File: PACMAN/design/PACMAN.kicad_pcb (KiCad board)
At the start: 2 copper layers, 47 x 57.2 mm, 8 parts, among them P1 RPi connector, P2 CO2, P3 DHT22, P4 Sonar, P5 PMS3003

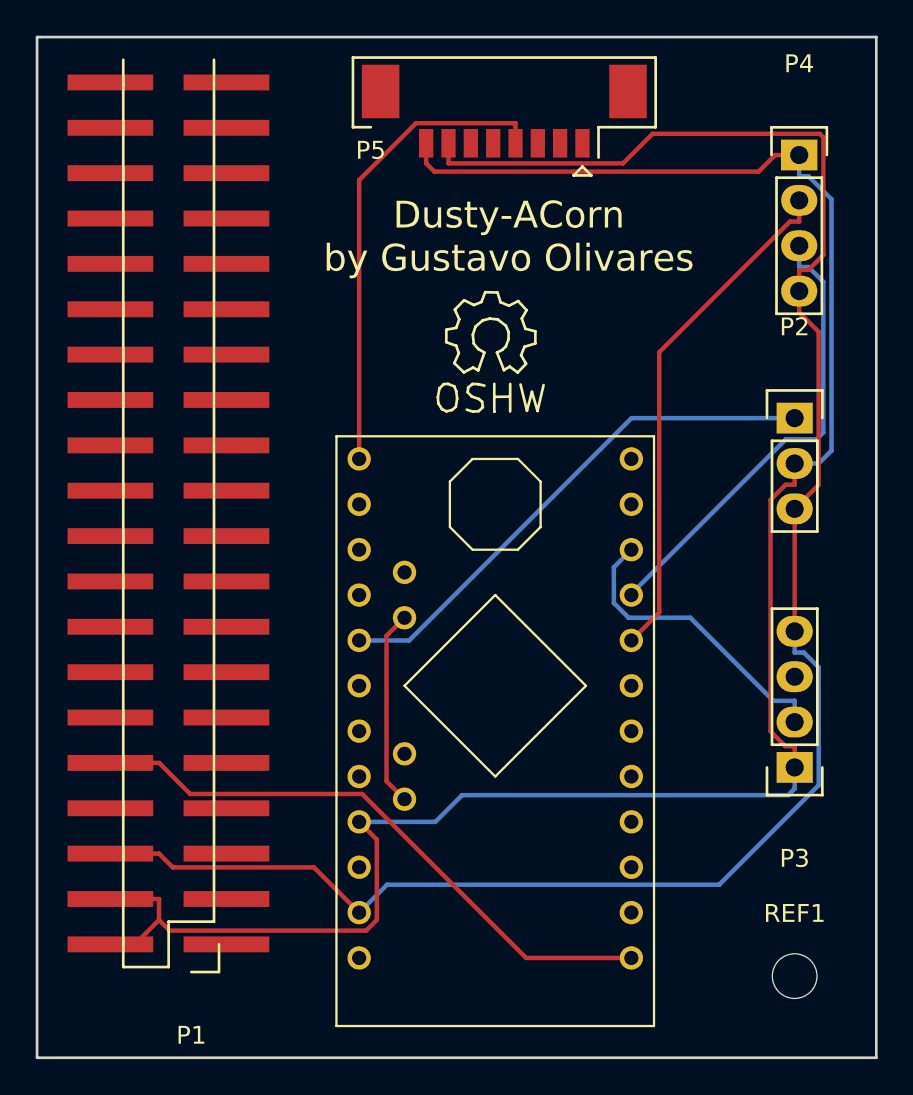
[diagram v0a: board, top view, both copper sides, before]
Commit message: Merging work at work to prepare deployment
Signed-off-by: Gustavo Olivares <guolivar@gmail.com>
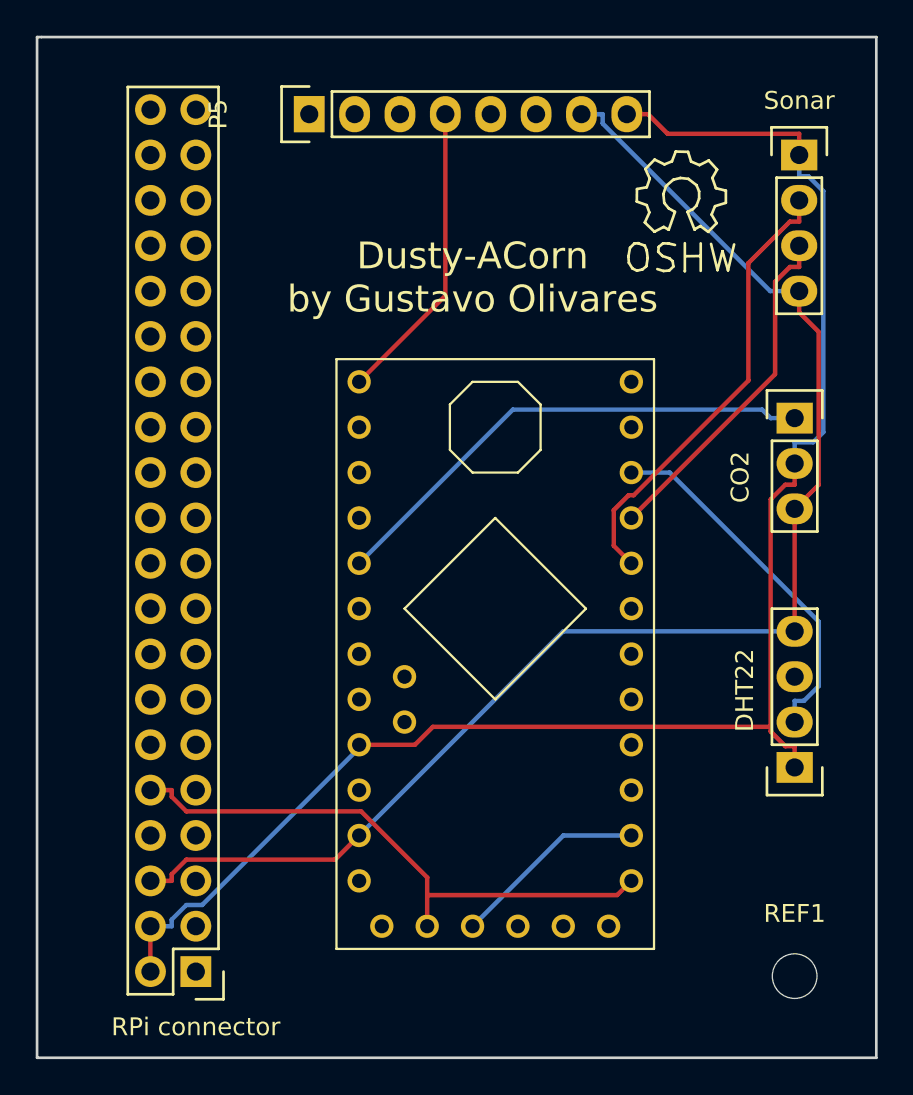
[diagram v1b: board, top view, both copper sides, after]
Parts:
- removed ??1: ARDUINO_PRO_MINI, arduino_pro_mini_V2:Halley-ARDUINO_PRO_MINI
- added MC1: ARDUINO_PRO_MINI, arduino:Halley-ARDUINO_PRO_MINI, F.Cu at (116.3, 111.5)
- P1: footprint headers:Pin_Header_Straight_2x20_SMD -> Pin_Headers:Pin_Header_Straight_2x20
- P5: footprint Connectors_Molex:Connector_Molex_PicoBlade_53261-0871 -> Pin_Headers:Pin_Header_Straight_1x08
- moved REF2 13.3 mm to (126.7, 84.6)
- moved P5 11.0 mm to (105.9, 80.0), turned to 90 degrees
- moved P1 1.55 mm to (99.6, 128.0)
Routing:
- net GND: track 105.9 -> 78.7 mm
- net +5V: track 113.4 -> 91.7 mm
- net Net-(??1-PadA5): track 11.0 -> 0.00 mm
- net Net-(MC1-PadRXI): track 0.00 -> 11.0 mm
- net /D10: track 26.8 -> 17.0 mm
- net /D6: track 25.9 -> 19.4 mm
- net /D7: track 17.0 -> 20.4 mm
- net /D5: track 28.8 -> 25.5 mm
- net /TX0: track 33.7 -> 32.2 mm
- net /A0: track 29.5 -> 28.1 mm
